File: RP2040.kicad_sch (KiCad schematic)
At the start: 1 part, among them U1 RP2040

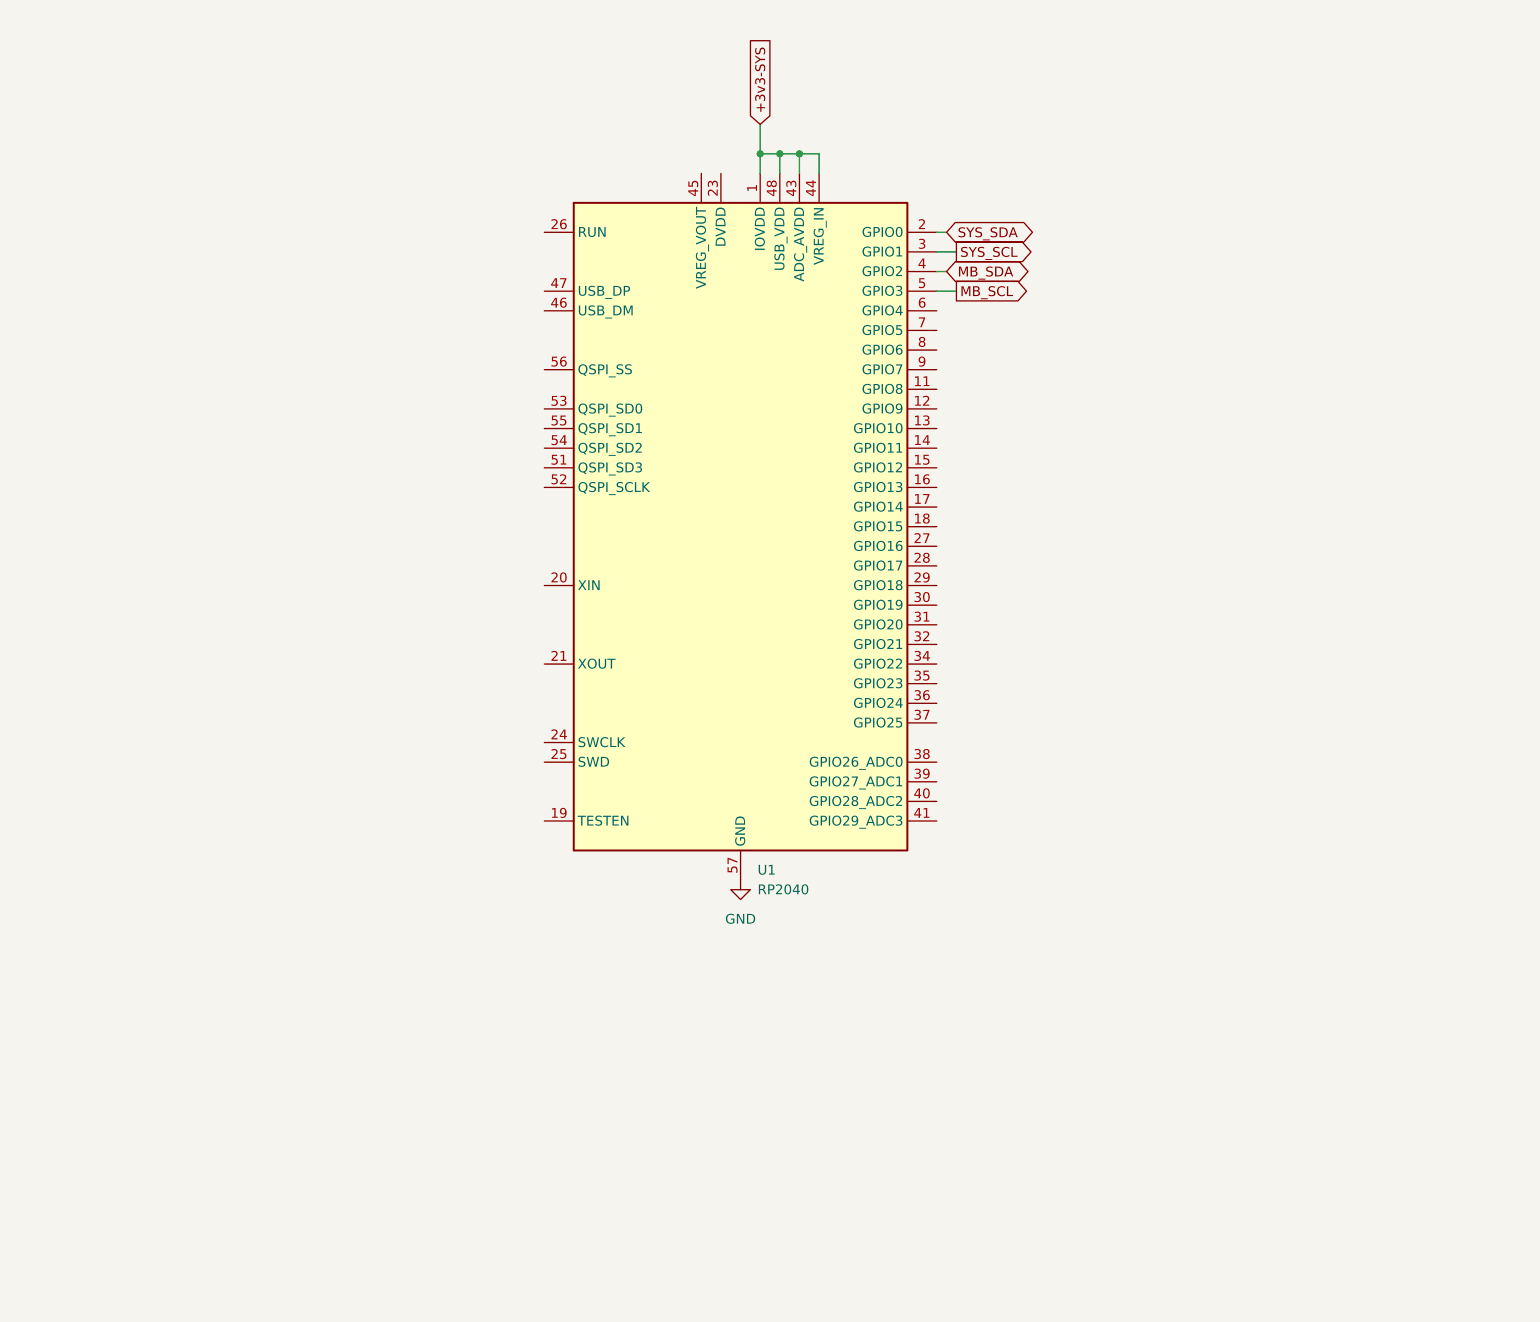
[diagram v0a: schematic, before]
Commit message: more rp2040 work
-BMS updates
- rp2040 updates
- add hardware design docs
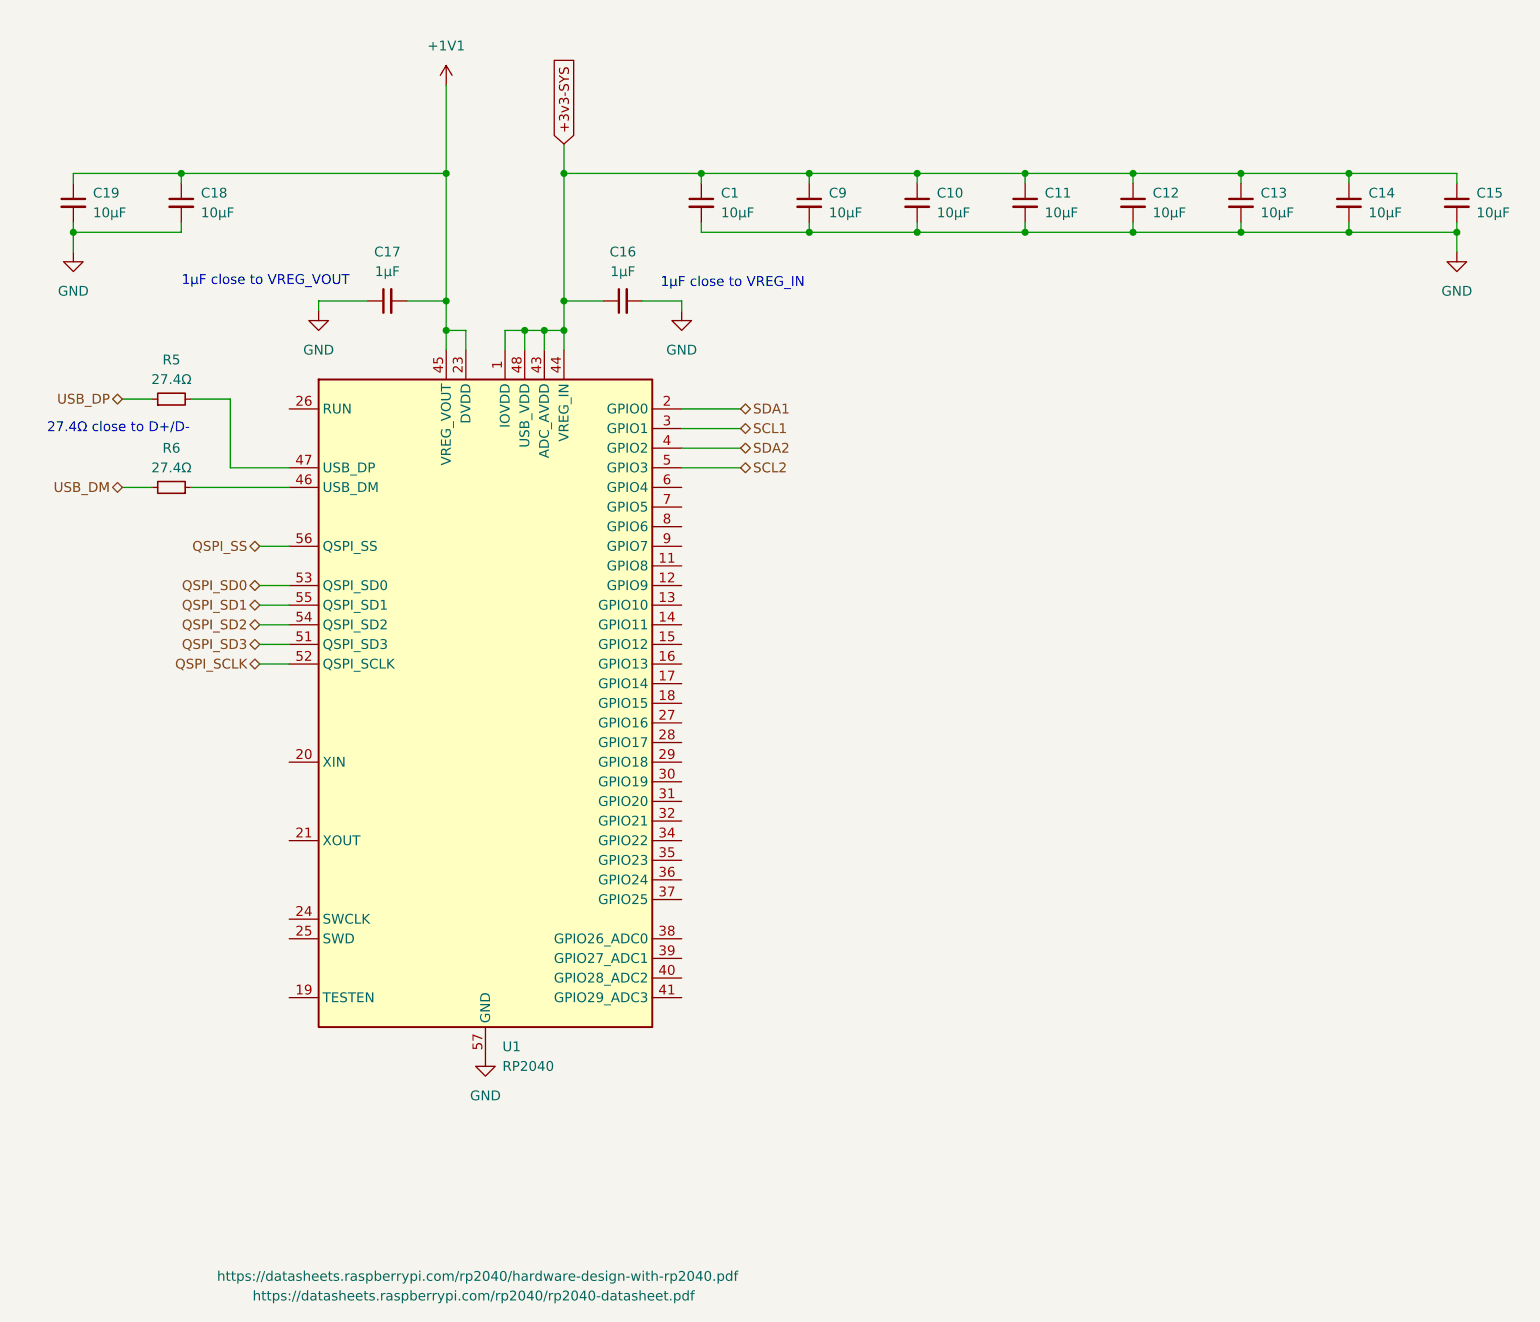
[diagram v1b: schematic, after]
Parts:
- added C1, C10, C11, C12, C13, C14, C15, C18, C19, C9: 10µF, symbol Device:C_Small
- added C16, C17: 1µF, symbol Device:C_Small
- added R5, R6: 27.4Ω, symbol Device:R_Small
- U1: Hardware Design Docs (none) -> https://datasheets.raspberrypi.com/rp2040/hardware-design-w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
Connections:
- net +3v3-SYS: now also C1.1, C10.1, C11.1, C12.1, C13.1, C14.1, C15.1, C16.1, C9.1
- net GND: now also C1.2, C10.2, C11.2, C12.2, C13.2, C14.2, C15.2, C16.2, C17.1, C18.2, C19.2, C9.2
- net +1V1: now reaches U1.23 (DVDD), U1.50 (DVDD)
- net +1V1: now also U1.45 (VREG_VOUT), C17.2, C18.1, C19.1
- net at U1.46 (USB_DM): now also R6.1
- net at U1.47 (USB_DP): now also R5.2
- net QSPI_SD3: now reaches U1.51 (QSPI_SD3)
- net QSPI_SCLK: now reaches U1.52 (QSPI_SCLK)
- net QSPI_SD0: now reaches U1.53 (QSPI_SD0)
- net QSPI_SD2: now reaches U1.54 (QSPI_SD2)
- net QSPI_SD1: now reaches U1.55 (QSPI_SD1)
- net QSPI_SS: now reaches U1.56 (QSPI_SS)
- net MB_SCL renamed SCL2
- net MB_SDA renamed SDA2
- net SYS_SCL renamed SCL1
- net SYS_SDA renamed SDA1
- new net USB_DM: R6.2
- new net USB_DP: R5.1
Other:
- note added: "1µF close to VREG_IN"
- note added: "1µF close to VREG_VOUT"
- note added: "27.4Ω close to D+/D-"
- moved on the sheet: U1
